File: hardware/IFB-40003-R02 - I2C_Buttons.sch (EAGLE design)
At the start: 32 parts, among them J10 CUT_JUMPER_2X, J3 CUTTABLE_JUMPER, J4 POGO_PAD, J5 POGO_PAD, J6 POGO_PAD, J7 POGO_PAD, J8 POGO_PAD, J9 POGO_PAD, SW1 PTS6455MM, SW2 PTS6455MM, SW3 PTS6455MM, SW4 PTS6455MM, SW5 PTS6455MM, U2 ATTINY841-MMHR

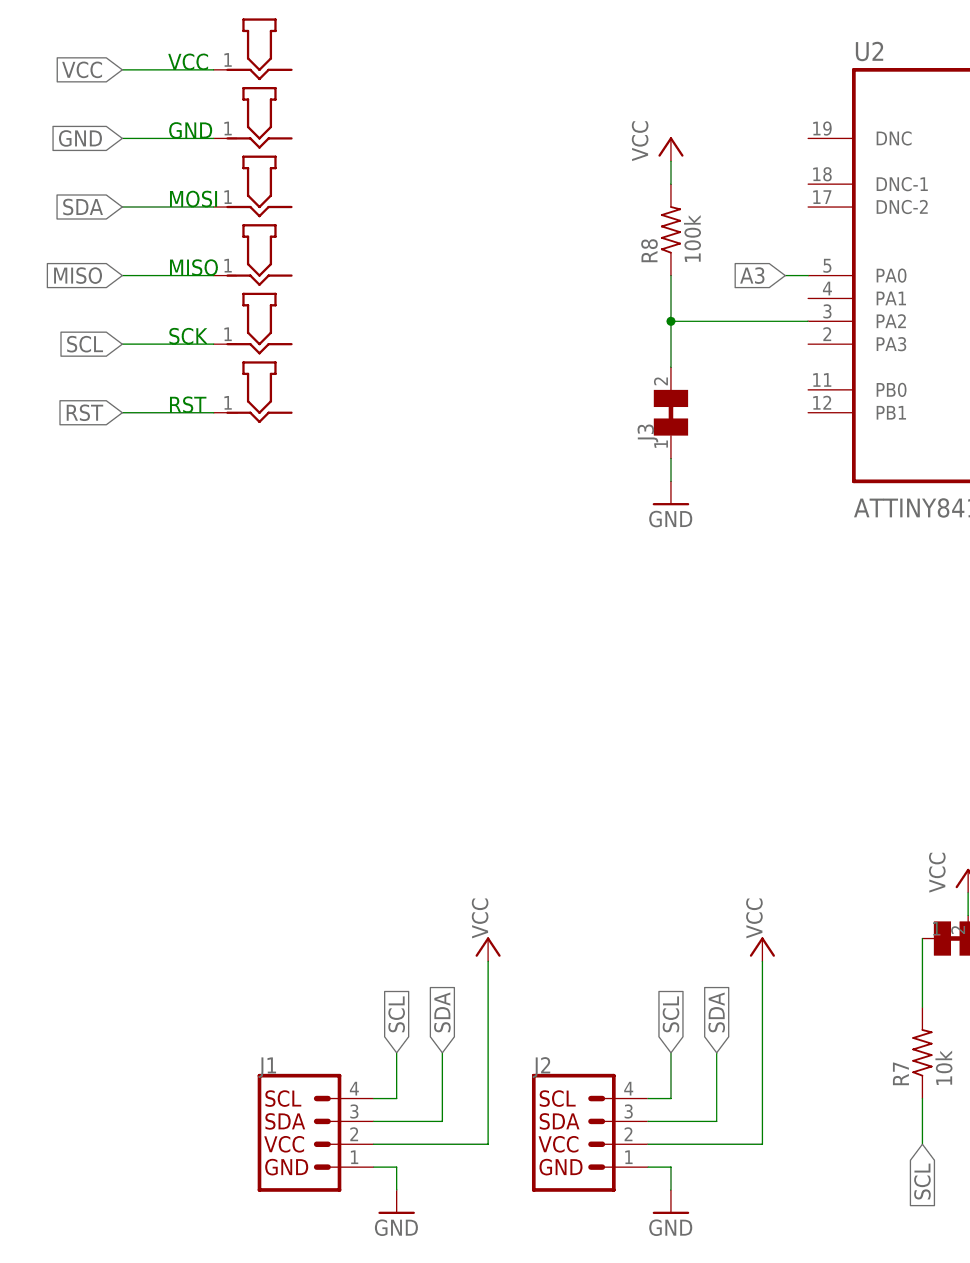
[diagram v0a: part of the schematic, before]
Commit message: updated hardware files
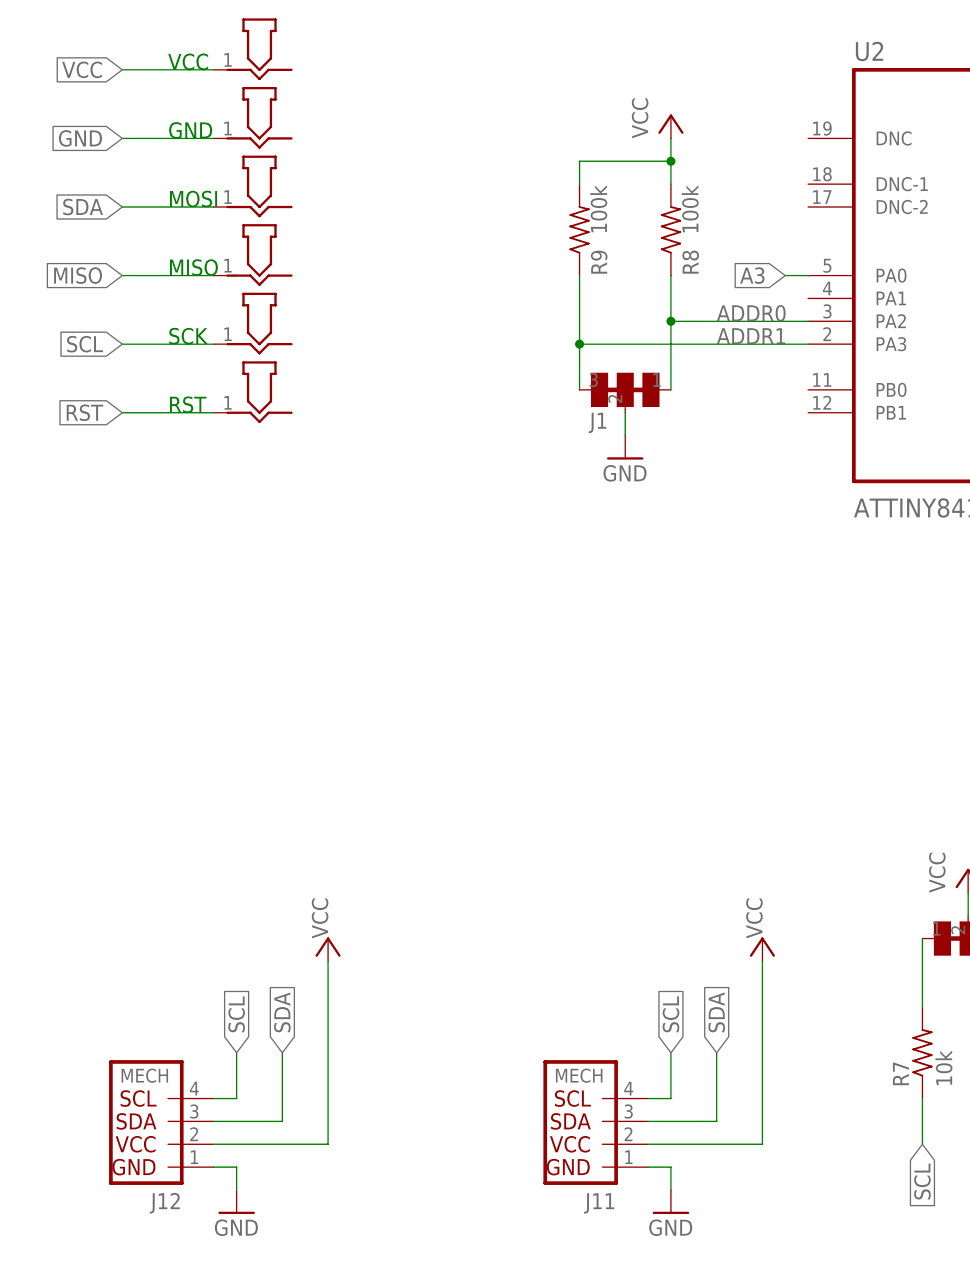
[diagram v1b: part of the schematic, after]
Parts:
- removed J2: (no value), SparkFun-Connectors:QWIIC_CONNECTORJS-1MM
- removed J3: CUTTABLE_JUMPER, PlayingWithFusion_Breakout-Lib:CUTTABLE_JUMPER
- added J11, J12: QWIICSIDE, PlayingWithFusion_JST:QWIICSIDE
- added R9: 100k, rcl:R-US_R0603
- J1: value (none) -> CUT_JUMPER_2X; device SparkFun-Connectors:QWIIC_CONNECTORJS-1MM -> PlayingWithFusion_Breakout-Lib:CUT_JUMPER_2X
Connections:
- removed net N$1: J3.2, R8.1, U2.PA2
- new net ADDR0: J1.1, R8.1, U2.PA2
- new net ADDR1: J1.3, R9.1, U2.PA3
- net GND: now also J1.2, J11.1, J12.1; no longer J1.GND, J2.GND, J3.1
- net SCL: now also J11.4, J12.4; no longer J1.SCL, J2.SCL
- net SDA: now also J11.3, J12.3; no longer J1.SDA, J2.SDA
- net VCC: now also J11.2, J12.2, R9.2; no longer J1.VCC, J2.VCC
